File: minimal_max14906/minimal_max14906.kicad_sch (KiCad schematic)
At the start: 106 parts, among them J1 CLP-114-02-G-D-BE, J10 TBP02R2-381-02BE, J11 TBP02R2-381-02BE, J12 CLP-103-02-G-D-BE, J2 TBP02R2-381-02BE, J3 TBP02R2-381-02BE, J4 CLP-102-02-G-D-BE, J5 CLP-102-02-G-D-BE, J6 CLP-102-02-G-D-BE, J7 CLP-102-02-G-D-BE, J8 CLP-102-02-G-D-BE, J9 CLP-102-02-G-D-BE, Q1 -60.0 V, Q2 -60.0 V, Q3 -60.0 V, Q4 -60.0 V, Q5 100 V, U1 ADUM1252AUA+, U2 MAX22441CAEE+, U3 MAX22442CAEE+, U4 ADUM1252AUA+, U5 MAX14906ATM+

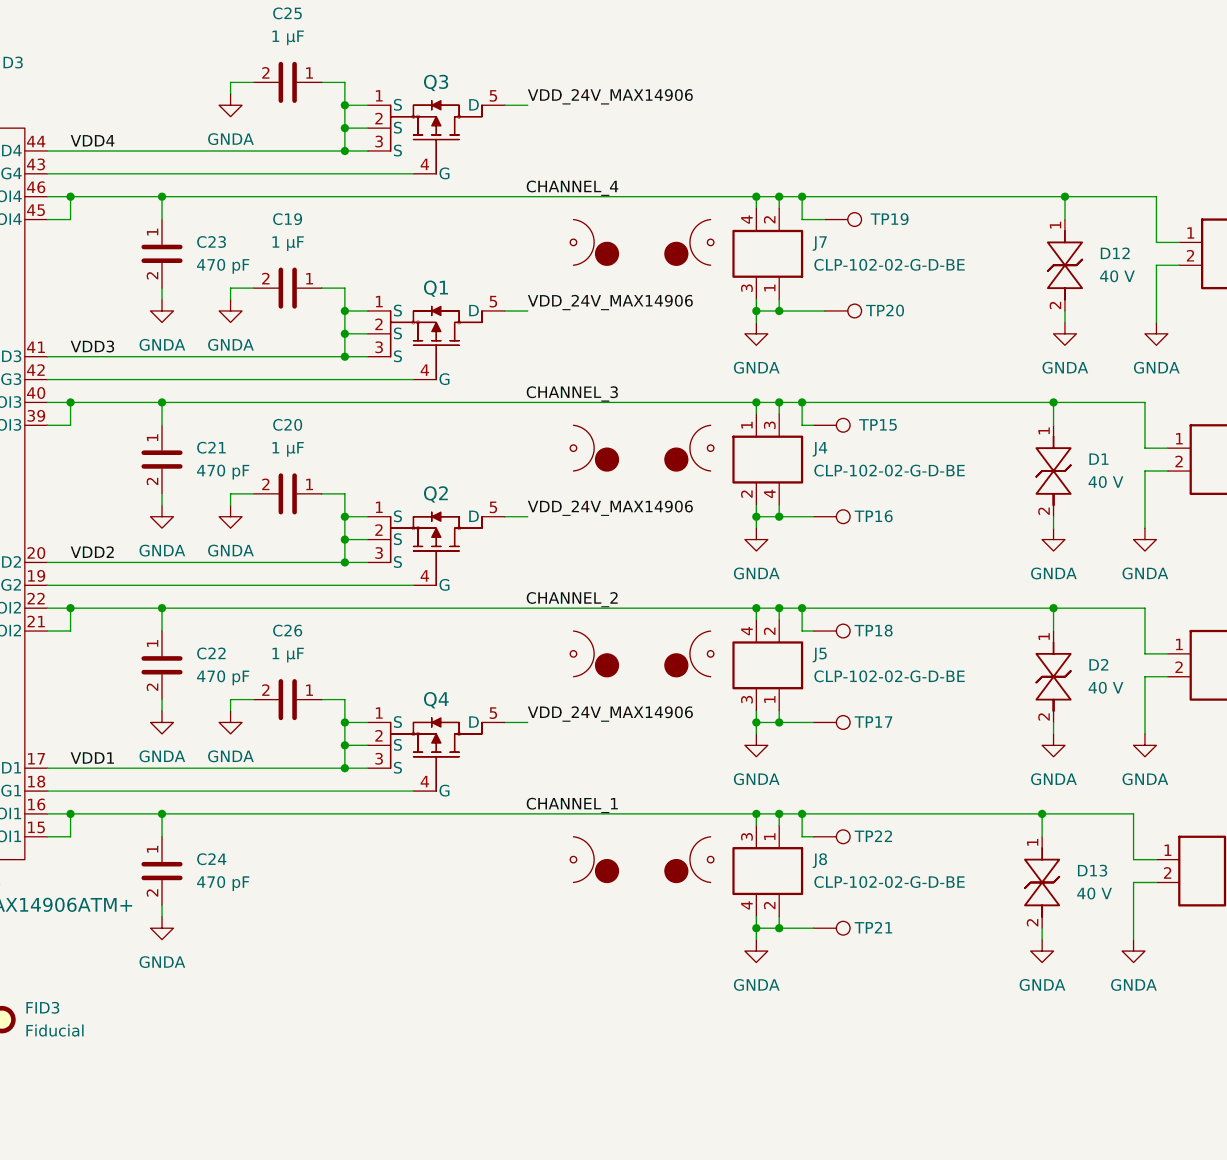
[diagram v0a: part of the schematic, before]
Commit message: development backup
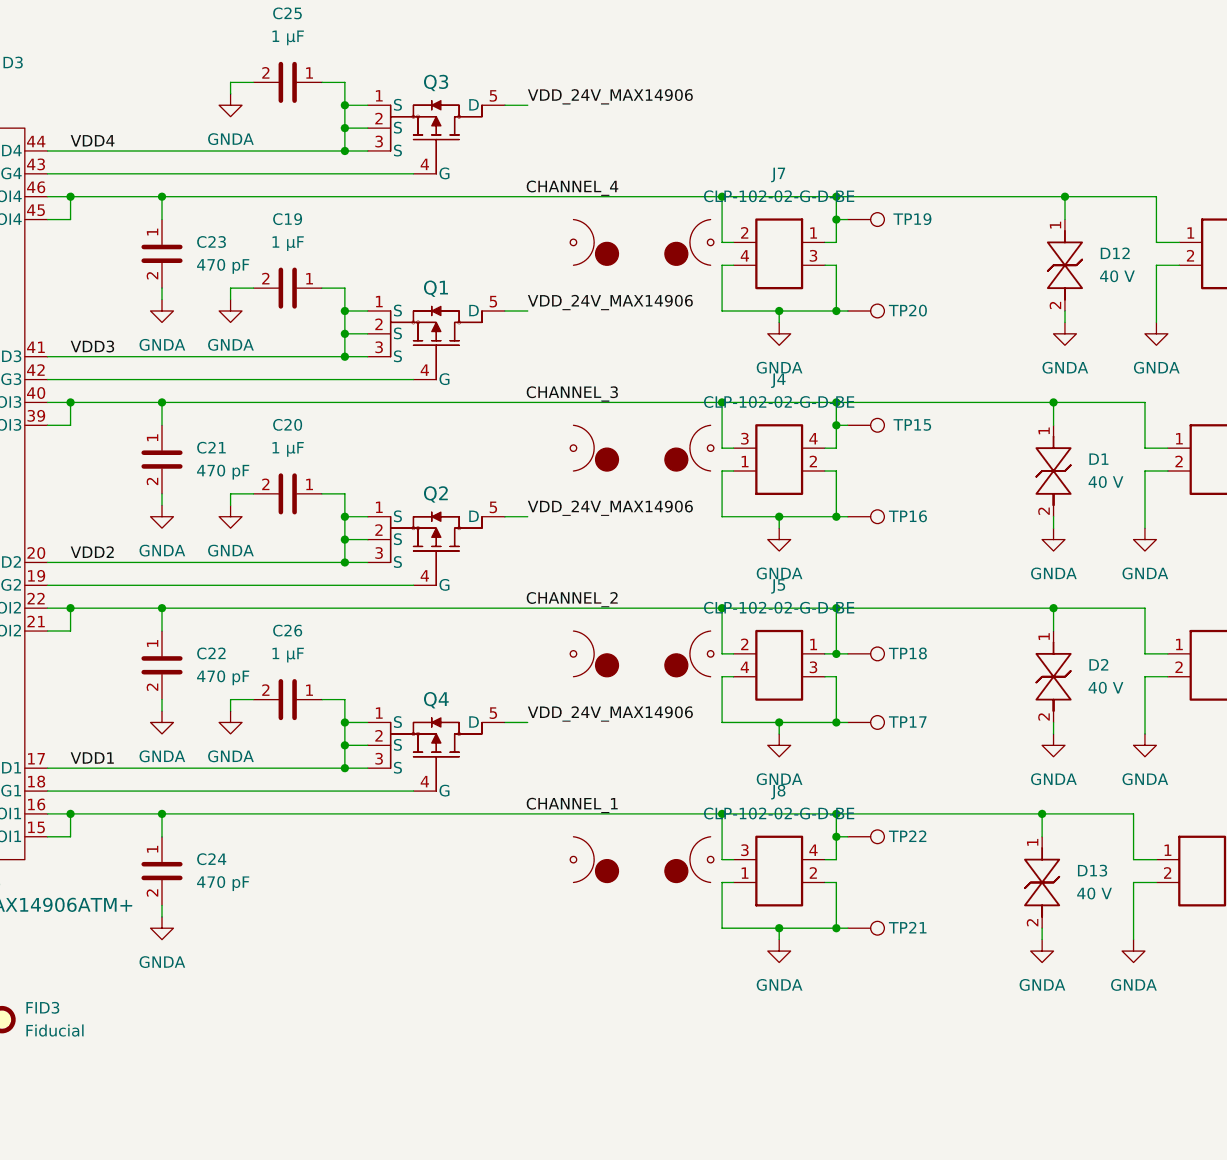
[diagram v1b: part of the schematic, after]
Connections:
- net CHANNEL_1: now also J8.4; no longer J8.1
- net CHANNEL_2: now also J5.1; no longer J5.4
- net CHANNEL_3: now also J4.4; no longer J4.1
- net CHANNEL_4: now also J7.1; no longer J7.4
- net GNDA: now also J4.1, J5.4, J7.4, J8.1; no longer J4.4, J5.1, J7.1, J8.4
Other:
- moved on the sheet: J4, J5, J7, J8, TP15, TP16, TP17, TP18, TP19, TP20, TP21, TP22
